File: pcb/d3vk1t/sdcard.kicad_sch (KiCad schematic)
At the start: 1 part, among them J1 Micro_SD_Card_Det

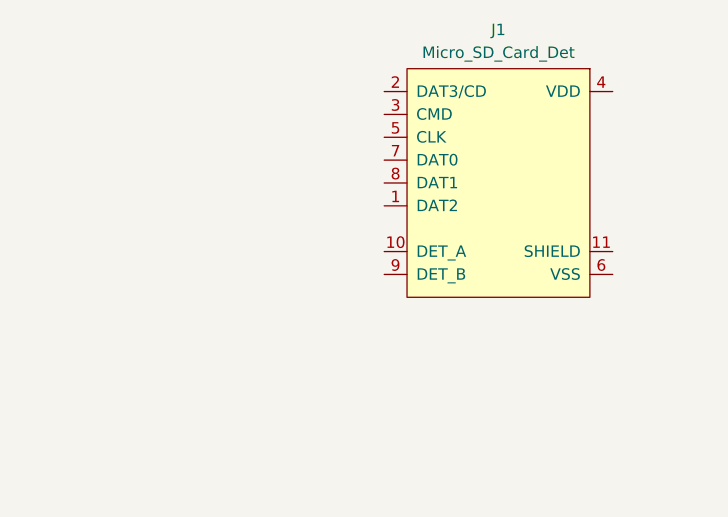
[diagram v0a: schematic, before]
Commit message: [update all schematics sheets]
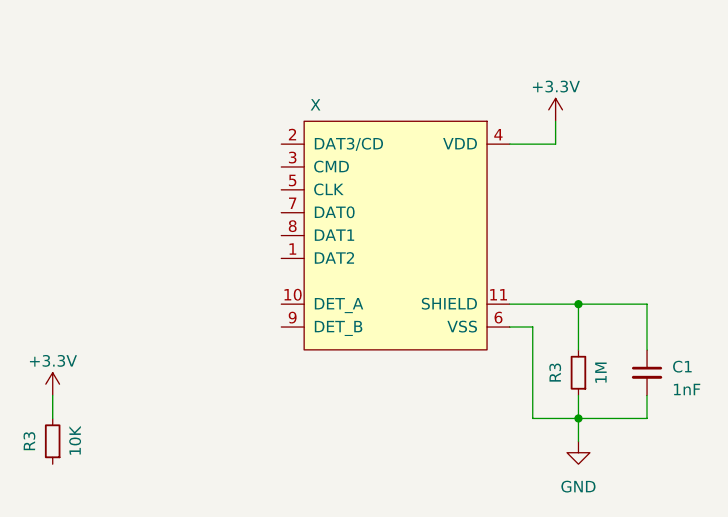
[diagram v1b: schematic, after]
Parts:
- added C1: 1nF, Capacitor_SMD:C_1206_3216Metric, symbol Device:C_Small
- added R3: 10K, Resistor_SMD:R_0402_1005Metric, symbol Device:R_Small
- added R3: 1M, Resistor_SMD:R_1206_3216Metric, symbol Device:R_Small
- renumbered J1 to X
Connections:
- net at X.11 (SHIELD): now also C1.1, R3.2
- net +3.3V: now reaches X.4 (VDD)
- net +3.3V: now also R3.2
- net GND: now reaches X.6 (VSS)
- net GND: now also C1.2, R3.1
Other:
- moved on the sheet: X
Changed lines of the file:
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@@
 (kicad_sch (version 20230121) (generator eeschema)
   (paper "A4")
-  (symbol (lib_id "db-sdcard:Micro_SD_Card_Det") (at 186.69 100.838 0) (mirror y) (unit 1)
-    (in_bom yes) (on_board yes) (dnp no) (fields_autoplaced)
-    (property "Reference" "J1" (at 186.69 83.82 0)
-      (effects (font (size 1.27 1.27)))
-    )
-    (property "Value" "Micro_SD_Card_Det" (at 186.69 86.36 0)
-      (effects (font (size 1.27 1.27)))
-    )
-    (property "Footprint" "db:microSD_SOFNG_TF-015" (at 134.62 83.058 0)
-      (effects (font (size 1.27 1.27)) hide)
-    )
-    (property "Datasheet" "https://www.hirose.com/product/en/download_file/key_name/DM3/category/Catalog/doc_file_id/49662/?file_category_id=4&item_id=195&is_series=1" (at 187.96 117.348 0)
+  (junction (at 195.58 127) (diameter 0) (color 0 0 0 0)
+  )
+  (junction (at 195.58 114.3) (diameter 0) (color 0 0 0 0)
+  )
+  (wire (pts (xy 137.16 124.46) (xy 137.16 127))
+    (stroke (width 0) (type default))
+  )
+  (wire (pts (xy 187.96 96.52) (xy 193.04 96.52))
+    (stroke (width 0) (type default))
+  )
+  (wire (pts (xy 195.58 127) (xy 190.5 127))
+    (stroke (width 0) (type default))
+  )
+  (wire (pts (xy 203.2 124.46) (xy 203.2 127))
+    (stroke (width 0) (type default))
+  )
+  (wire (pts (xy 193.04 93.98) (xy 193.04 96.52))
+    (stroke (width 0) (type default))
+  )
+  (wire (pts (xy 195.58 124.46) (xy 195.58 127))
+    (stroke (width 0) (type default))
+  )
+  (wire (pts (xy 195.58 127) (xy 195.58 129.54))
+    (stroke (width 0) (type default))
+  )
+  (wire (pts (xy 187.96 116.84) (xy 190.5 116.84))
+    (stroke (width 0) (type default))
+  )
+  (wire (pts (xy 203.2 114.3) (xy 203.2 119.38))
+    (stroke (width 0) (type default))
+  )
+  (wire (pts (xy 190.5 116.84) (xy 190.5 127))
+    (stroke (width 0) (type default))
+  )
+  (wire (pts (xy 195.58 114.3) (xy 203.2 114.3))
+    (stroke (width 0) (type default))
+  )
+  (wire (pts (xy 195.58 119.38) (xy 195.58 114.3))
+    (stroke (width 0) (type default))
+  )
+  (wire (pts (xy 195.58 114.3) (xy 187.96 114.3))
+    (stroke (width 0) (type default))
+  )
+  (wire (pts (xy 203.2 127) (xy 195.58 127))
+    (stroke (width 0) (type default))
+  )
+  (symbol (lib_id "power:+3.3V") (at 193.04 93.98 0) (unit 1)
+    (in_bom yes) (on_board yes) (dnp no) (fields_autoplaced)
+    (property "Reference" "#PWR02" (at 193.04 97.79 0)
+      (effects (font (size 1.27 1.27)) hide)
+    )
+    (property "Value" "+3.3V" (at 193.04 90.17 0)
+      (effects (font (size 1.27 1.27)))
+    )
+    (property "Footprint" "" (at 193.04 93.98 0)
+      (effects (font (size 1.27 1.27)) hide)
+    )
+    (property "Datasheet" "" (at 193.04 93.98 0)
+      (effects (font (size 1.27 1.27)) hide)
+    )
+    (pin "1")
+    (instances
+      (project "d3vk1t"
+        (path "/4ea523ae-7c45-478e-a9cc-6f4833d1a9d5/0c7e2350-c710-4f8b-bffc-99ae7438d4de"
+          (reference "#PWR02") (unit 1)
+        )
+        (path "/4ea523ae-7c45-478e-a9cc-6f4833d1a9d5/41f8e312-86c0-4917-8944-524577576fad"
+          (reference "#PWR014") (unit 1)
+        )
+        (path "/4ea523ae-7c45-478e-a9cc-6f4833d1a9d5/aea6c2ba-3179-4867-b0ce-0dd87f8d3618"
+          (reference "#PWR027") (unit 1)
+        )
+      )
+    )
+  )
+  (symbol (lib_id "power:+3.3V") (at 137.16 124.46 0) (unit 1)
+    (in_bom yes) (on_board yes) (dnp no) (fields_autoplaced)
+    (property "Reference" "#PWR02" (at 137.16 128.27 0)
+      (effects (font (size 1.27 1.27)) hide)
+    )
+    (property "Value" "+3.3V" (at 137.16 120.65 0)
+      (effects (font (size 1.27 1.27)))
+    )
+    (property "Footprint" "" (at 137.16 124.46 0)
+      (effects (font (size 1.27 1.27)) hide)
+    )
+    (property "Datasheet" "" (at 137.16 124.46 0)
+      (effects (font (size 1.27 1.27)) hide)
+    )
+    (pin "1")
+    (instances
+      (project "d3vk1t"
+        (path "/4ea523ae-7c45-478e-a9cc-6f4833d1a9d5/0c7e2350-c710-4f8b-bffc-99ae7438d4de"
+          (reference "#PWR02") (unit 1)
+        )
+        (path "/4ea523ae-7c45-478e-a9cc-6f4833d1a9d5/41f8e312-86c0-4917-8944-524577576fad"
+          (reference "#PWR012") (unit 1)
+        )
+        (path "/4ea523ae-7c45-478e-a9cc-6f4833d1a9d5/aea6c2ba-3179-4867-b0ce-0dd87f8d3618"
+          (reference "#PWR050") (unit 1)
+        )
+      )
+    )
+  )
+  (symbol (lib_id "db-sdcard:Micro_SD_Card_Det") (at 175.26 106.68 0) (mirror y) (unit 1)
+    (in_bom yes) (on_board yes) (dnp no)
+    (property "Reference" "X" (at 166.37 92.202 0)
+      (effects (font (size 1.27 1.27)))
+    )
+    (property "Value" "Micro_SD_Card_Det" (at 175.26 92.202 0)
+      (effects (font (size 1.27 1.27)) hide)
+    )
+    (property "Footprint" "db:microSD_SOFNG_TF-015" (at 123.19 88.9 0)
+      (effects (font (size 1.27 1.27)) hide)
+    )
+    (property "Datasheet" "https://www.hirose.com/product/en/download_file/key_name/DM3/category/Catalog/doc_file_id/49662/?file_category_id=4&item_id=195&is_series=1" (at 176.53 123.19 0)
       (effects (font (size 1.27 1.27)) hide)
     )
@@
       (project "d3vk1t"
         (path "/4ea523ae-7c45-478e-a9cc-6f4833d1a9d5/aea6c2ba-3179-4867-b0ce-0dd87f8d3618"
-          (reference "J1") (unit 1)
-        )
-      )
+          (reference "X") (unit 1)
+        )
+      )
+    )
+  )
+  (symbol (lib_id "Device:C_Small") (at 203.2 121.92 0) (unit 1)
+    (in_bom yes) (on_board yes) (dnp no) (fields_autoplaced)
+    (property "Reference" "C1" (at 205.994 121.2913 0)
+      (effects (font (size 1.27 1.27)) (justify left))
+    )
+    (property "Value" "1nF" (at 205.994 123.8313 0)
+      (effects (font (size 1.27 1.27)) (justify left))
+    )
+    (property "Footprint" "Capacitor_SMD:C_1206_3216Metric" (at 203.2 121.92 0)
+      (effects (font (size 1.27 1.27)) hide)
+    )
+    (property "Datasheet" "~" (at 203.2 121.92 0)
+      (effects (font (size 1.27 1.27)) hide)
+    )
+    (pin "1")
+    (pin "2")
+    (instances
+      (project "d3vk1t"
+        (path "/4ea523ae-7c45-478e-a9cc-6f4833d1a9d5/0c7e2350-c710-4f8b-bffc-99ae7438d4de"
+          (reference "C1") (unit 1)
+        )
+        (path "/4ea523ae-7c45-478e-a9cc-6f4833d1a9d5/41f8e312-86c0-4917-8944-524577576fad"
+          (reference "C12") (unit 1)
+        )
+        (path "/4ea523ae-7c45-478e-a9cc-6f4833d1a9d5/fd7cf4b0-4d20-445a-8ab6-186a5df83da1"
+          (reference "C13") (unit 1)
+        )
+        (path "/4ea523ae-7c45-478e-a9cc-6f4833d1a9d5/aea6c2ba-3179-4867-b0ce-0dd87f8d3618"
+          (reference "C14") (unit 1)
+        )
+      )
+    )
+  )
+  (symbol (lib_id "power:GND") (at 195.58 129.54 0) (unit 1)
+    (in_bom yes) (on_board yes) (dnp no) (fields_autoplaced)
+    (property "Reference" "#PWR026" (at 195.58 135.89 0)
+      (effects (font (size 1.27 1.27)) hide)
+    )
+    (property "Value" "GND" (at 195.58 134.62 0)
+      (effects (font (size 1.27 1.27)))
+    )
+    (property "Footprint" "" (at 195.58 129.54 0)
+      (effects (font (size 1.27 1.27)) hide)
+    )
+    (property "Datasheet" "" (at 195.58 129.54 0)
+      (effects (font (size 1.27 1.27)) hide)
+    )
+    (pin "1")
+    (instances
+      (project "d3vk1t"
+        (path "/4ea523ae-7c45-478e-a9cc-6f4833d1a9d5/aea6c2ba-3179-4867-b0ce-0dd87f8d3618"
+          (reference "#PWR026") (unit 1)
+        )
+      )
+    )
+  )
+  (symbol (lib_id "Device:R_Small") (at 137.16 129.54 180) (unit 1)
+    (in_bom yes) (on_board yes) (dnp no)
+    (property "Reference" "R3" (at 134.62 129.54 90)
+      (effects (font (size 1.27 1.27)))
+    )
+    (property "Value" "10K" (at 139.7 129.54 90)
+      (effects (font (size 1.27 1.27)))
+    )
+    (property "Footprint" "Resistor_SMD:R_0402_1005Metric" (at 137.16 129.54 0)
+      (effects (font (size 1.27 1.27)) hide)
+    )
+    (property "Datasheet" "~" (at 137.16 129.54 0)
+      (effects (font (size 1.27 1.27)) hide)
+    )
+    (pin "1")
+    (pin "2")
+    (instances
+      (project "d3vk1t"
+        (path "/4ea523ae-7c45-478e-a9cc-6f4833d1a9d5/41f8e312-86c0-4917-8944-524577576fad"
+          (reference "R3") (unit 1)
+        )
+        (path "/4ea523ae-7c45-478e-a9cc-6f4833d1a9d5/aea6c2ba-3179-4867-b0ce-0dd87f8d3618"
+          (reference "R15") (unit 1)
+        )
+      )
+    )
+  )
+  (symbol (lib_id "Device:R_Small") (at 195.58 121.92 180) (unit 1)
+    (in_bom yes) (on_board yes) (dnp no)
+    (property "Reference" "R3" (at 193.04 121.92 90)
+      (effects (font (size 1.27 1.27)))
+    )
+    (property "Value" "1M" (at 198.12 121.92 90)
+      (effects (font (size 1.27 1.27)))
+    )
+    (property "Footprint" "Resistor_SMD:R_1206_3216Metric" (at 195.58 121.92 0)
+      (effects (font (size 1.27 1.27)) hide)
+    )
+    (property "Datasheet" "~" (at 195.58 121.92 0)
+      (effects (font (size 1.27 1.27)) hide)
+    )
+    (pin "1")
+    (pin "2")
+    (instances
+      (project "d3vk1t"
+        (path "/4ea523ae-7c45-478e-a9cc-6f4833d1a9d5/41f8e312-86c0-4917-8944-524577576fad"
+          (reference "R3") (unit 1)
+        )
+        (path "/4ea523ae-7c45-478e-a9cc-6f4833d1a9d5/fd7cf4b0-4d20-445a-8ab6-186a5df83da1"
+          (reference "R6") (unit 1)
+        )
+        (path "/4ea523ae-7c45-478e-a9cc-6f4833d1a9d5/aea6c2ba-3179-4867-b0ce-0dd87f8d3618"
+          (reference "R9") (unit 1)
+        )
+      )
